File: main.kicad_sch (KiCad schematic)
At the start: 220 parts, among them J1 DC-005-5A-2.5-SMT, J2 Conn_01x07_Pin, J3 Conn_01x04_Pin, J4 TYPE-C-31-M-31, J5 Conn_01x11_Pin, J6 Conn_01x11_Pin, J7 Conn_01x11_Pin, Q1 STL6P3LLH6, Q2 STL6P3LLH6, SW1 TS-1088-AR02016, SW2 TS-1088-AR02016, U1 AP1117-33, U10 TPS55289RYQR, U11 TPS55289RYQR, U12 LMR16030PDDAR, U13 LMR16030PDDAR, U2 ESP32-C3, U3 STUSB4500QTR, U4 PCA9555PW, U5 W25Q128JVS, U6 INA180A2, U7 INA180A2, U8 INA180A2, U9 INA180A2, Y1 X322540MPB4SI

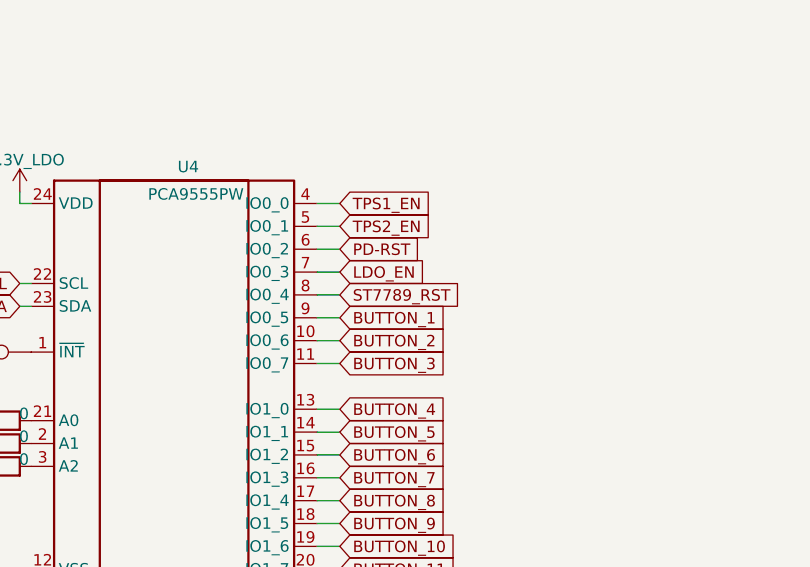
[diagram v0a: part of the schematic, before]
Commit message: Finished rev0
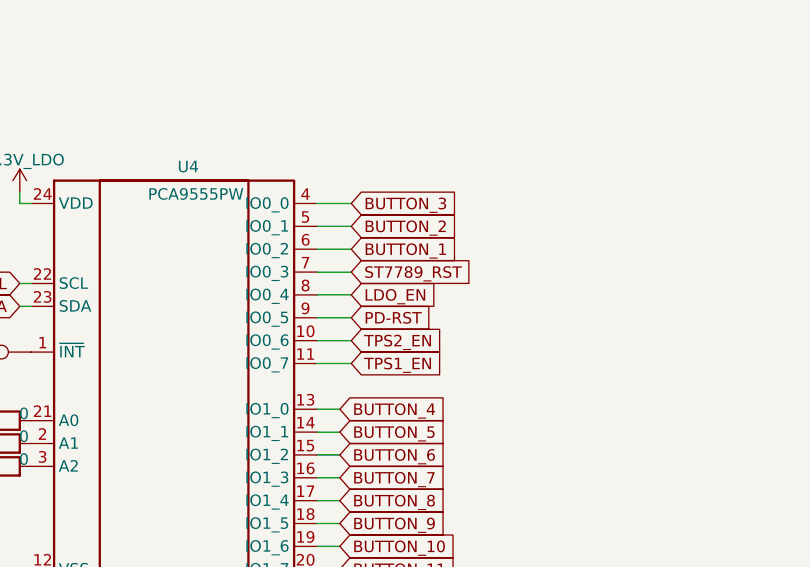
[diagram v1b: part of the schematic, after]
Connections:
- net BUTTON_1: now also U4.6 (IO0_2); no longer U4.9 (IO0_5)
- net BUTTON_2: now also U4.5 (IO0_1); no longer U4.10 (IO0_6)
- net BUTTON_3: now also U4.4 (IO0_0); no longer U4.11 (IO0_7)
- net LDO_EN: now also U4.8 (IO0_4); no longer U4.7 (IO0_3)
- net PD-RST: now also U4.9 (IO0_5); no longer U4.6 (IO0_2)
- net ST7789_RST: now also U4.7 (IO0_3); no longer U4.8 (IO0_4)
- net TPS1_EN: now also U4.11 (IO0_7); no longer U4.4 (IO0_0)
- net TPS2_EN: now also U4.10 (IO0_6); no longer U4.5 (IO0_1)
